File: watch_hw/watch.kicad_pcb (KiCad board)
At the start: 6 copper layers, 38 x 40 mm, 61 parts, among them J1 2130830005, J2 FH19C-7S-0.5SH, M1 VZ43FC1B5640005L, SW1 TL6340AF160Q, SW2 TL6340AF160Q, U1 NRF52833-QDAA, U2 nPM1100-QD, U3 MAX17048G+, U4 BMA456, U5 DRV2603, U6 LIS3MDL, Y1 32MHz, Y2 32.768kHz

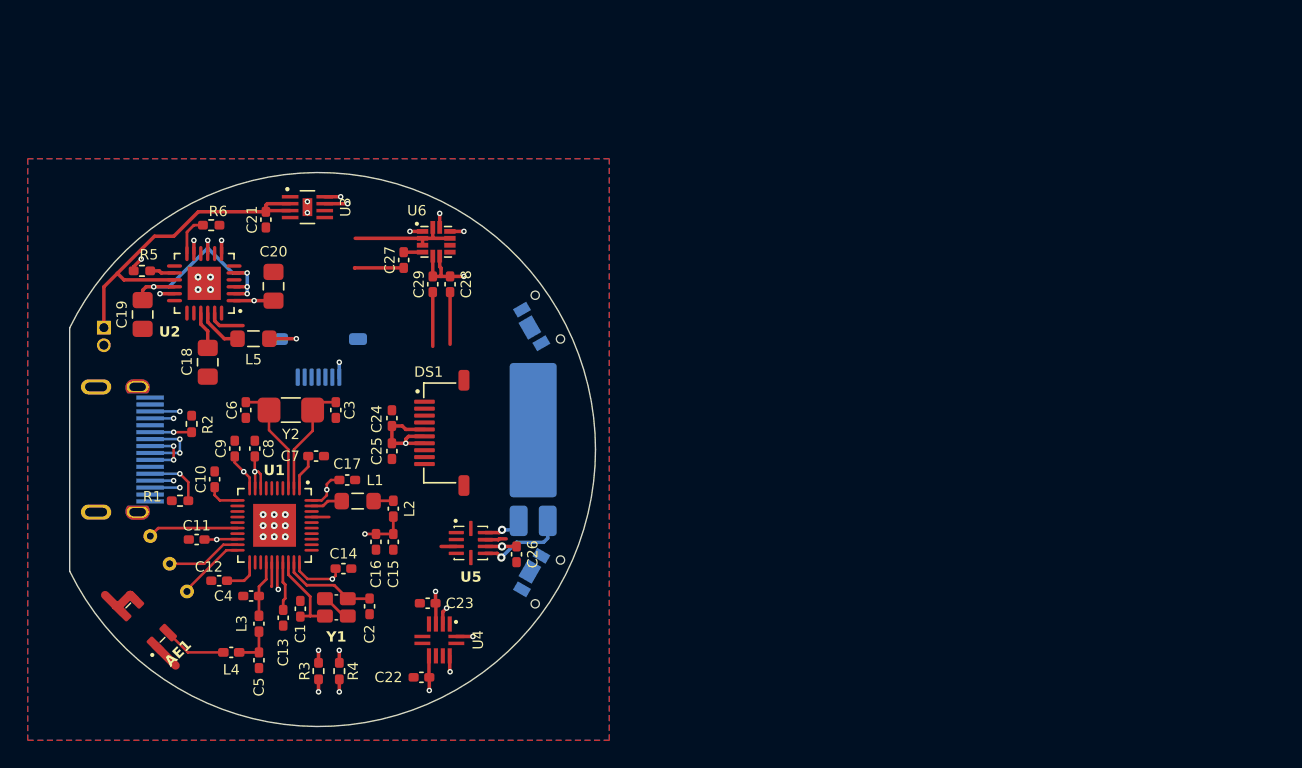
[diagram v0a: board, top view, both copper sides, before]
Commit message: Start watch v1 layout
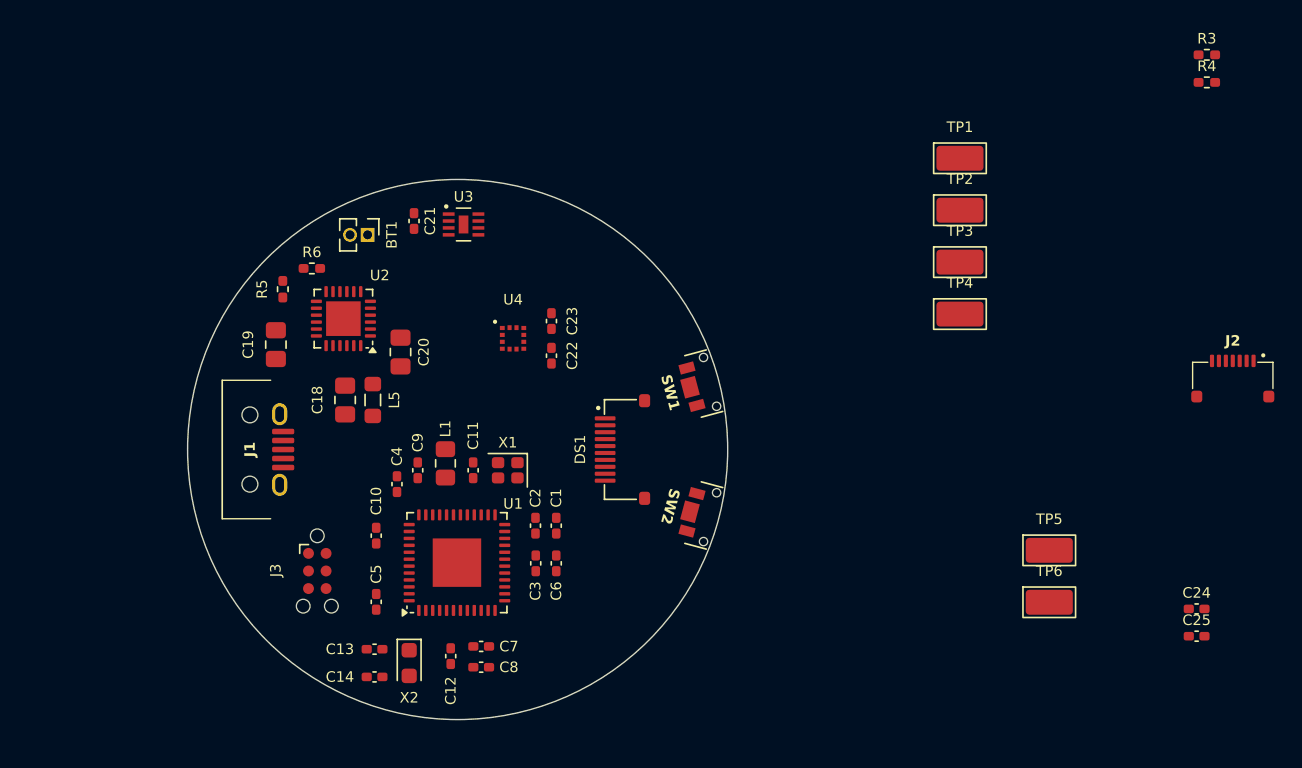
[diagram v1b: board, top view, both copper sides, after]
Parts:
- removed AE1: 2450AT18D0100001, watch:ANTENNA_2450AT18D0100001
- removed C15, C17, C28: 1uF, Capacitor_SMD:C_0402_1005Metric_Pad0.74x0.62mm_HandSolder
- removed C16: 47nF, Capacitor_SMD:C_0402_1005Metric_Pad0.74x0.62mm_HandSolder
- removed C26, C27, C29: 0.1uF, Capacitor_SMD:C_0402_1005Metric_Pad0.74x0.62mm_HandSolder
- removed L2: 15nH, Inductor_SMD:L_0402_1005Metric_Pad0.77x0.64mm_HandSolder
- removed L3: 4.7nF, Inductor_SMD:L_0402_1005Metric_Pad0.77x0.64mm_HandSolder
- removed L4: 2.2nH, Inductor_SMD:L_0402_1005Metric_Pad0.77x0.64mm_HandSolder
- removed M1: VZ43FC1B5640005L, watch:VZ43FC1B5640005L
- removed R1, R2: 5.1k, Resistor_SMD:R_0402_1005Metric_Pad0.72x0.64mm_HandSolder
- removed the REF** at (140.0, 100.0)
- removed U5: DRV2603, watch:DRV2603RUN
- removed U6: LIS3MDL, watch:LIS3MDLTR
- removed Y1: 32MHz, watch:XTAL_ECX-1637B2
- removed Y2: 32.768kHz, watch:XTAL_SC32S
- added J3: Conn_ARM_SWD_TagConnect_TC2030-NL, Connector:Tag-Connect_TC2030-IDC-NL_2x03_P1.27mm_Vertical, F.Cu at (139.9, 108.8)
- added TP4: TestPoint, TestPoint:TestPoint_Keystone_5015_Micro_Mini, F.Cu at (186.3, 90.2)
- added TP5: TestPoint, TestPoint:TestPoint_Keystone_5015_Micro_Mini, F.Cu at (192.7, 107.3)
- added TP6: TestPoint, TestPoint:TestPoint_Keystone_5015_Micro_Mini, F.Cu at (192.7, 111.0)
- added X1: NX2016SA-32M, Crystal:Crystal_SMD_2016-4Pin_2.0x1.6mm, F.Cu at (153.6, 101.5)
- added X2: NX2012_32K768, Crystal:Crystal_SMD_2012-2Pin_2.0x1.2mm_HandSoldering, F.Cu at (146.5, 115.4)
- BT1, SW1, SW2: moved to F.Cu
- C1: value 9pF -> 100nF
- C10: value 4.7uF -> 100nF
- C11: value 0.1uF -> 4.7uF
- C12: value 820pF -> 100nF
- C13: value 100pF -> 10pF
- C14: value 0.1uF -> 10pF
- C2: value 9pF -> 100pF
- C3: value 10pF -> 100nF
- C4: value 1pF -> 100nF
- C5: value 1.2pF -> 100nF
- C6: value 10pF -> 4.7uF
- C7: value 0.1uF -> 10nF
- C8: value 4.7uF -> 1uF
- J1: value 2130830005 -> USB_B_Micro; footprint watch:MOLEX_2130830005 -> watch:UJ2-MIBH-4-SMT-TR-67; moved to F.Cu
- J2: value FH19C-7S-0.5SH -> FH19C-7S-0.5SH(10); moved to F.Cu
- L1: footprint Inductor_SMD:L_0805_2012Metric_Pad1.05x1.20mm_HandSolder -> Inductor_SMD:L_0805_2012Metric_Pad1.15x1.40mm_HandSolder
- TP1: value SWDCLK -> TestPoint; footprint TestPoint:TestPoint_THTPad_D1.0mm_Drill0.5mm -> TestPoint:TestPoint_Keystone_5015_Micro_Mini; moved to F.Cu
- TP2: value SWDIO -> TestPoint; footprint TestPoint:TestPoint_THTPad_D1.0mm_Drill0.5mm -> TestPoint:TestPoint_Keystone_5015_Micro_Mini; moved to F.Cu
- TP3: value RESET -> TestPoint; footprint TestPoint:TestPoint_THTPad_D1.0mm_Drill0.5mm -> TestPoint:TestPoint_Keystone_5015_Micro_Mini; moved to F.Cu
- U1: value NRF52833-QDAA -> STM32WB55CGUx; footprint watch:nRF52833-QD -> Package_DFN_QFN:QFN-48-1EP_7x7mm_P0.5mm_EP3.5x3.5mm
- U2: footprint watch:nPM1100-QD -> Package_DFN_QFN:QFN-24-1EP_4x4mm_P0.5mm_EP2.5x2.5mm
- moved R3 78.1 mm to (204.1, 71.5), turned to 0 degrees
- moved R4 75.7 mm to (204.1, 73.5), turned to 0 degrees
- moved J2 66.0 mm to (206.0, 94.9)
- moved TP1 64.0 mm to (186.3, 79.0), turned to 0 degrees
- moved TP2 62.5 mm to (186.3, 82.7), turned to 0 degrees
- moved TP3 61.7 mm to (186.3, 86.5), turned to 0 degrees
- moved C24 59.7 mm to (203.4, 111.5), turned to 0 degrees
- moved C25 59.6 mm to (203.4, 113.5), turned to 0 degrees
- moved C22 25.1 mm to (156.8, 93.2), turned to 90 degrees
- moved C6 25.0 mm to (157.1, 108.2), turned to -90 degrees
- moved C8 22.7 mm to (151.7, 115.7), turned to 0 degrees
- moved U4 22.4 mm to (154.0, 92.0), turned to 0 degrees
- moved C23 22.2 mm to (156.8, 90.7), turned to -90 degrees
- moved C11 20.6 mm to (151.1, 101.5), turned to -90 degrees
- moved BT1 20.2 mm to (143.5, 84.5), turned to -90 degrees
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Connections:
- C1 pad 1: GND -> VDD
- C1 pad 2: Net-(U1-XC1) -> GND
- C10 pad 1: /SoC/DECUSB -> VDD
- C11 pad 1: VDD -> Net-(U1-VFBSMPS)
- C12 pad 1: /SoC/DEC5 -> /SoC/NRST
- C13 pad 1: /SoC/DEC3 -> /SoC/OSC32_IN
- C14 pad 1: VDD -> /SoC/OSC32_OUT
- C2 pad 1: GND -> VDD
- C2 pad 2: Net-(U1-XC2) -> GND
- C3 pad 1: GND -> VDD
- C3 pad 2: Net-(U1-P0.00/XL1) -> GND
- C4 pad 1: Net-(U1-ANT) -> VDD
- C5 pad 1: Net-(C5-Pad1) -> VDD
- C6 pad 1: GND -> VDD
- C6 pad 2: Net-(U1-P0.01/XL2) -> GND
- C7 pad 1: /SoC/DEC1 -> VDD
- C9 pad 1: VBUS -> VDD
- L1 pad 1: Net-(U1-DCC) -> Net-(U1-VLXSMPS)
- L1 pad 2: Net-(L1-Pad2) -> Net-(U1-VFBSMPS)
- TP1 pad 1: Net-(U1-SWDCLK) -> GND
- TP2 pad 1: Net-(U1-SWDIO) -> VDD
- TP3 pad 1: Net-(U1-P0.18/~{RESET}) -> /Power/VBAT
- U1 pad 1: /SoC/DEC1 -> VDD
- U1 pad 10: VBUS -> unconnected-(U1-PA1-Pad10)
- U1 pad 11: /SoC/DECUSB -> unconnected-(U1-PA2-Pad11)
- U1 pad 12: /USB_D_N -> unconnected-(U1-PA3-Pad12)
- U1 pad 13: /USB_D_P -> unconnected-(U1-PA4-Pad13)
- U1 pad 16: Net-(U1-P0.18/~{RESET}) -> unconnected-(U1-PA7-Pad16)
- U1 pad 18: VDD -> unconnected-(U1-PA9-Pad18)
- U1 pad 19: Net-(U1-SWDIO) -> unconnected-(U1-PB2-Pad19)
- U1 pad 2: Net-(U1-P0.00/XL1) -> /SoC/OSC32_IN
- U1 pad 20: Net-(U1-SWDCLK) -> VDD
- U1 pad 21: /SoC/DEC5 -> unconnected-(U1-RF1-Pad21)
- U1 pad 22: unconnected-(U1-P0.09/NFC1-Pad22) -> GND
- U1 pad 23: unconnected-(U1-P0.10/NFC2-Pad23) -> VDD
- U1 pad 24: Net-(U1-ANT) -> /SoC/OSC_OUT
- U1 pad 25: GND -> /SoC/OSC_IN
- U1 pad 26: /SoC/DEC6 -> unconnected-(U1-AT0-Pad26)
- U1 pad 27: /SoC/DEC3 -> unconnected-(U1-AT1-Pad27)
- U1 pad 28: Net-(U1-XC1) -> unconnected-(U1-PB0-Pad28)
- U1 pad 29: Net-(U1-XC2) -> unconnected-(U1-PB1-Pad29)
- U1 pad 3: Net-(U1-P0.01/XL2) -> /SoC/OSC32_OUT
- U1 pad 30: VDD -> unconnected-(U1-PE4-Pad30)
- U1 pad 31: unconnected-(U1-P0.03/AIN1-Pad31) -> Net-(U1-VFBSMPS)
- U1 pad 32: unconnected-(U1-P0.02/AIN0-Pad32) -> GND
- U1 pad 33: unconnected-(U1-P0.28/AIN4-Pad33) -> Net-(U1-VLXSMPS)
- U1 pad 34: unconnected-(U1-P0.29/AIN5-Pad34) -> VDD
- U1 pad 35: unconnected-(U1-P0.30/AIN6-Pad35) -> VDD
- U1 pad 37: GND -> unconnected-(U1-PA11-Pad37)
- U1 pad 38: /SoC/DEC4 -> unconnected-(U1-PA12-Pad38)
- U1 pad 39: Net-(U1-DCC) -> /SoC/SWDIO
- U1 pad 41: GND -> /SoC/SWCLK
- U1 pad 7: unconnected-(U1-P0.11-Pad7) -> /SoC/NRST
- U1 pad 9: VDD -> unconnected-(U1-PA0-Pad9)
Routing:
- net VDD: track 50.3 -> 0.00 mm, vias 16 -> 0
- net GND: track 38.7 -> 0.00 mm, vias 18 -> 0
- net /Power/VBAT: track 25.3 -> 0.00 mm
- net /Power/VSYS: track 17.6 -> 0.00 mm, vias 5 -> 0
- net /SoC/DEC6: track 13.2 -> 0.00 mm, vias 2 -> 0
- net VBUS: track 10.9 -> 0.00 mm, vias 6 -> 0
- net Net-(U1-P0.01/XL2): track 8.14 -> 0.00 mm
- net Net-(U1-P0.00/XL1): track 8.12 -> 0.00 mm
- net Net-(U1-XC2): track 6.98 -> 0.00 mm
- net Net-(U1-P0.18/~{RESET}): track 6.54 -> 0.00 mm
- net Net-(M1--): track 6.45 -> 0.00 mm, vias 1 -> 0
- net Net-(U1-XC1): track 6.32 -> 0.00 mm
- net Net-(U1-SWDIO): track 5.47 -> 0.00 mm
- net /USB_D_N: track 5.02 -> 0.00 mm, vias 2 -> 0
- net Net-(U1-SWDCLK): track 4.96 -> 0.00 mm
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- removed copper zone on B.Cu, net GND
- removed copper zone on F.Cu, net GND
- removed copper zone on In1.Cu, net GND
- removed copper zone on In4.Cu, net GND
- removed copper zone on In2.Cu, net VBUS
- removed copper zone on In2.Cu, net VDD
- removed copper zone on In3.Cu, net VDD
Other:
- board size 38 x 40 mm -> 39 x 39 mm
